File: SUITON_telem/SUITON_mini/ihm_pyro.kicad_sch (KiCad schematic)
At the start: 19 parts, among them Q3 BSS138, U11 74HC2G14GW_125

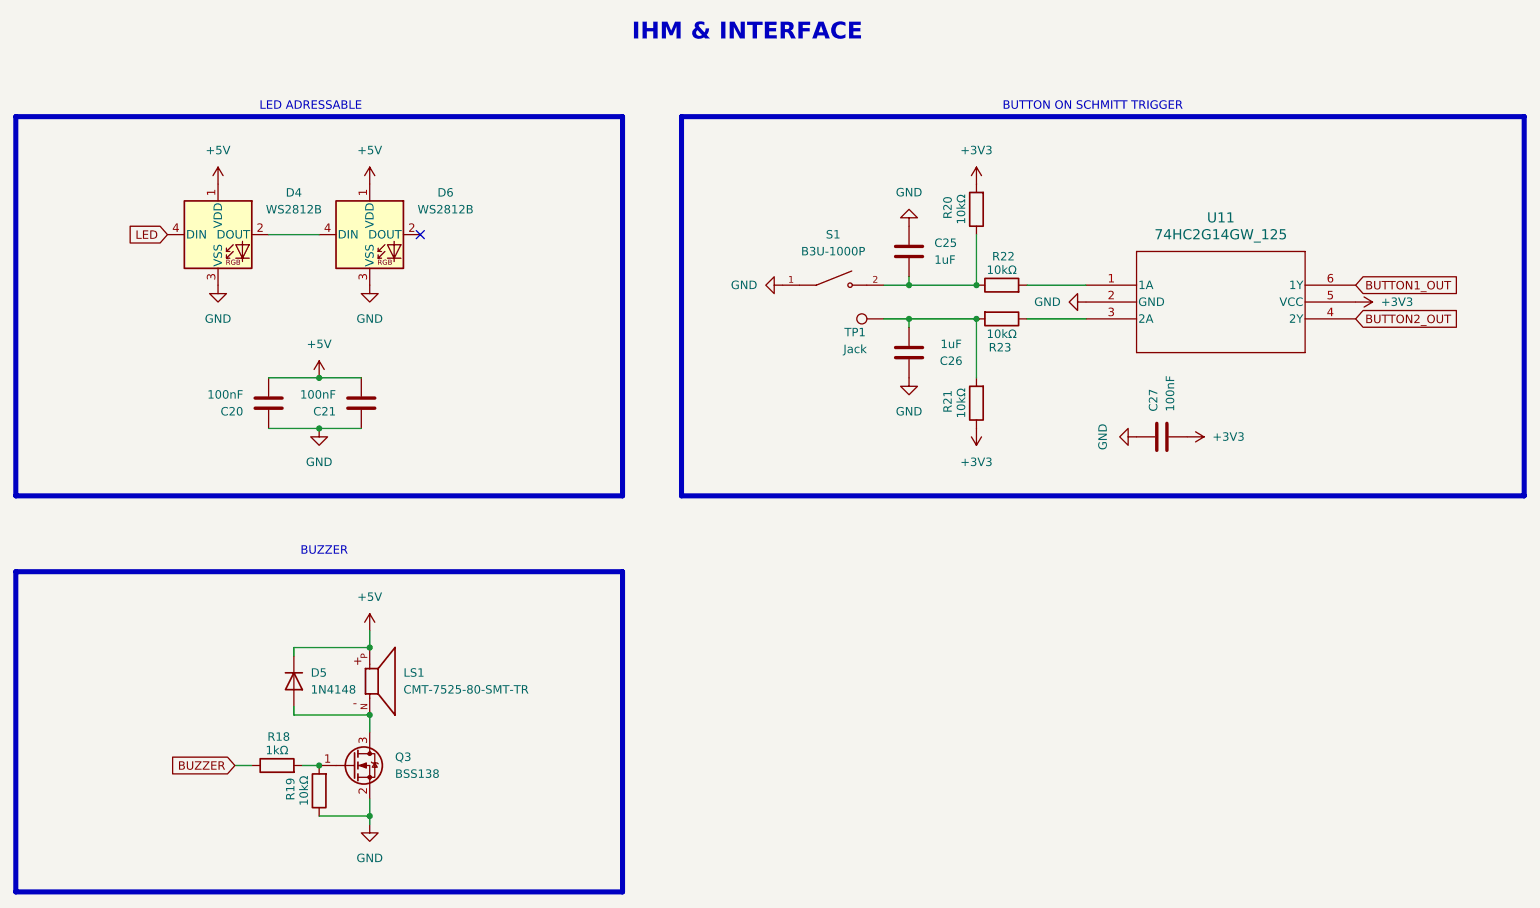
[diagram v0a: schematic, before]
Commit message: New rf module
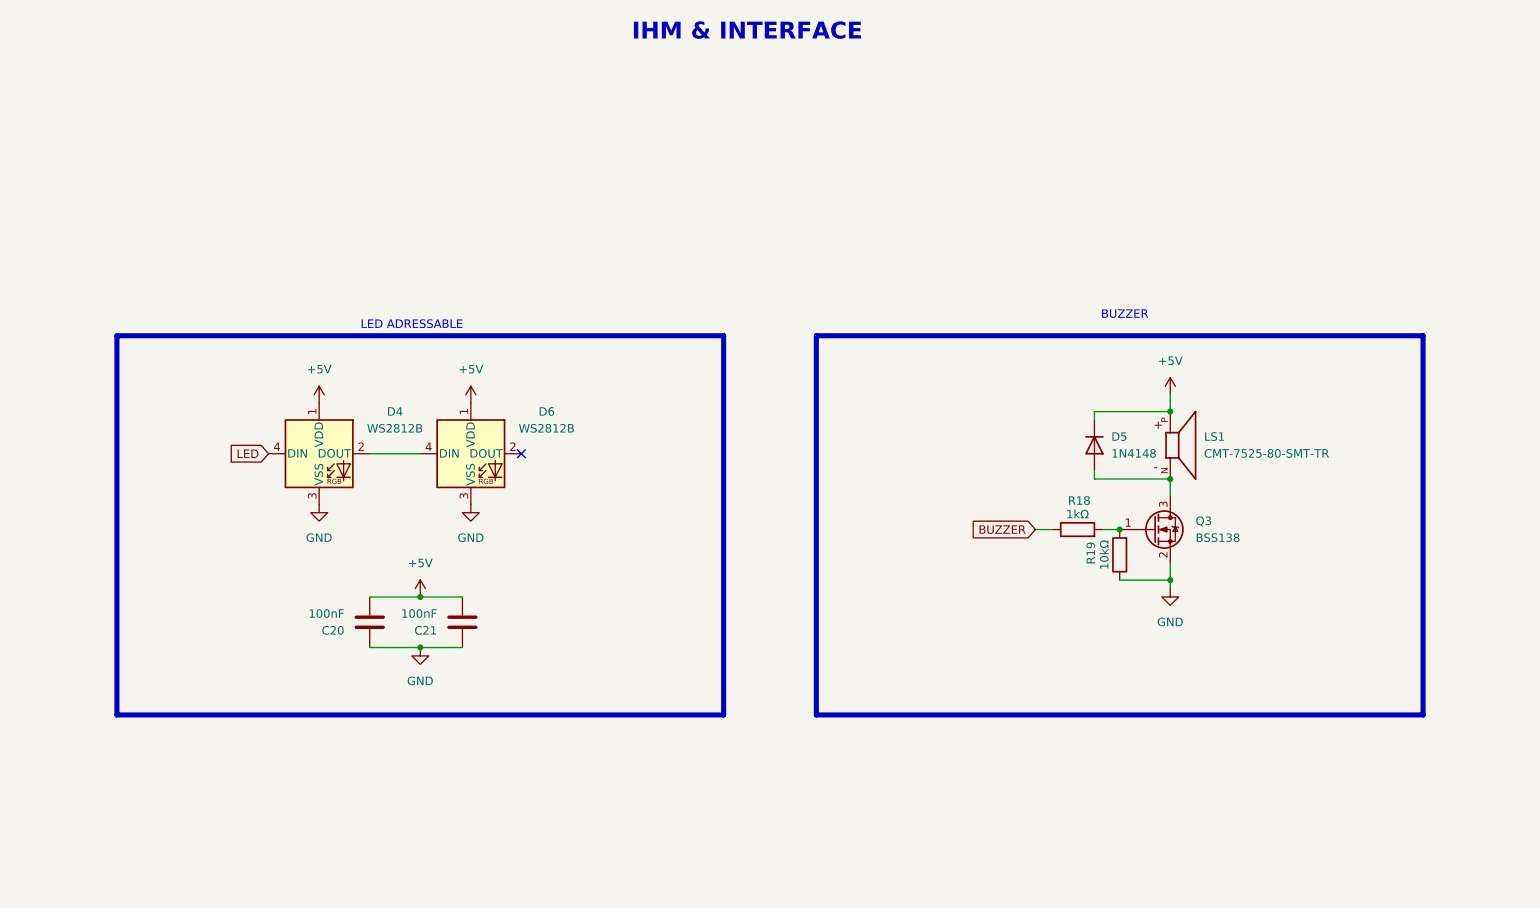
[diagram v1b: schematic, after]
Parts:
- removed C25, C26: 1uF, Capacitor_SMD:C_0603_1608Metric, symbol Device:C
- removed C27: 100nF, Capacitor_SMD:C_0603_1608Metric, symbol Device:C
- removed R20, R21, R22, R23: 10kΩ, symbol Device:R
- removed S1: B3U-1000P, B3U-1000P:SW_B3U-1000P, symbol B3U-1000P:B3U-1000P
- removed TP1: Jack, symbol Connector:TestPoint
- removed U11: 74HC2G14GW_125, TSSOP6_SOT363-2_NEX, symbol 2026-10-04_17-37-41:74HC2G14GW_125
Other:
- note removed: "BUTTON ON SCHMITT TRIGGER"
- moved on the sheet: C20, C21, D4, D5, D6, LS1, Q3, R18, R19
